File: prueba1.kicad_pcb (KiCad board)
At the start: 2 copper layers, 98.5 x 97 mm, 20 parts, among them J1 GY_63, J2 BMI_270, J3 CMPS2, J4 SHT21, J5 ATGM336H, J7 Cargador, J8 KG200Z, J9 BATERIA, Q1 MCP1702-3302E_TO, U1 TEMP_BAT, U2 DC-DC_STEP_UP

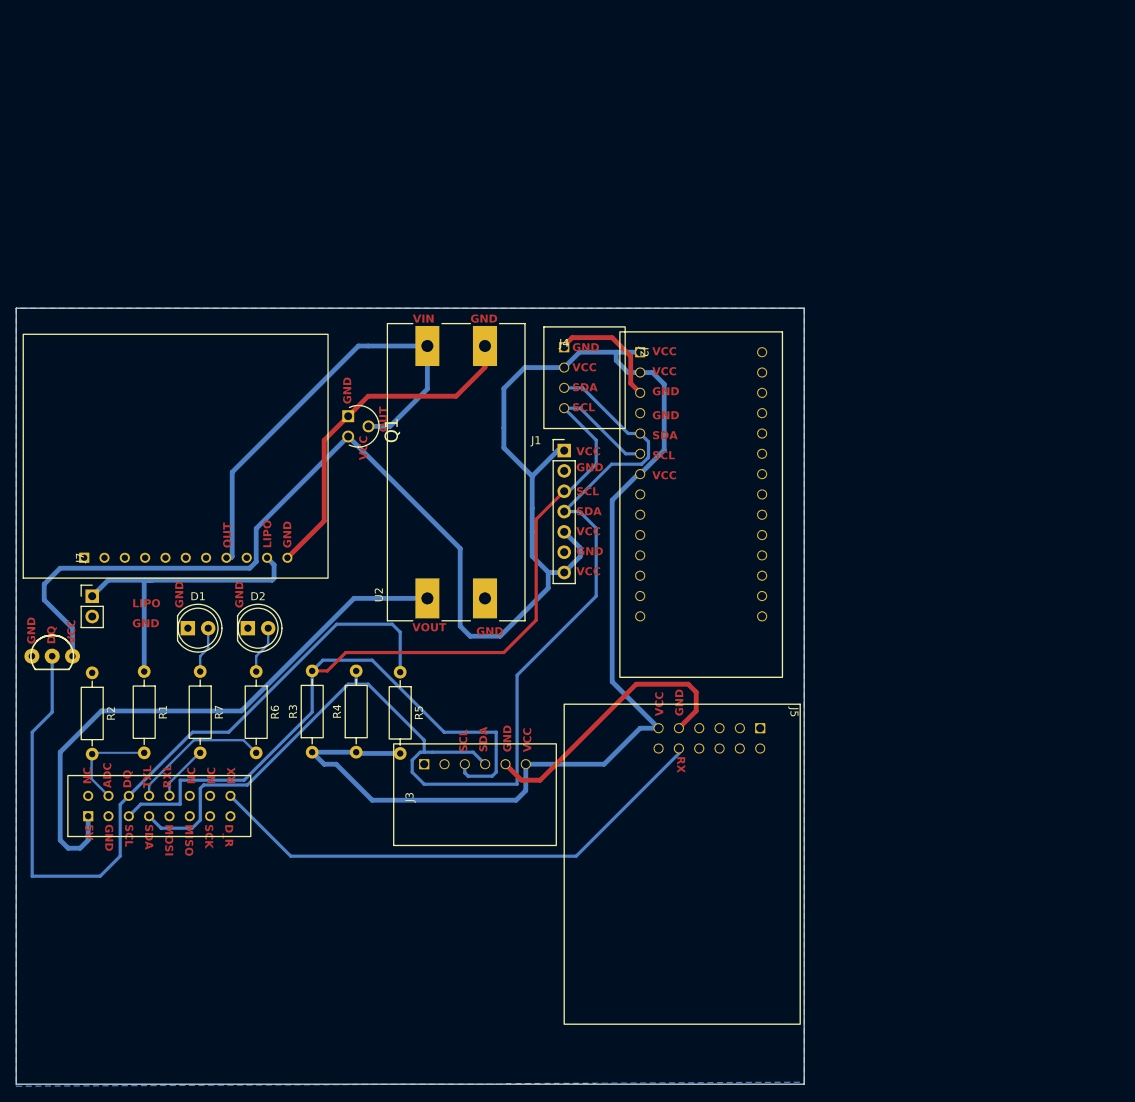
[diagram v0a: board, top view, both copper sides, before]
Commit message: pcb terminada
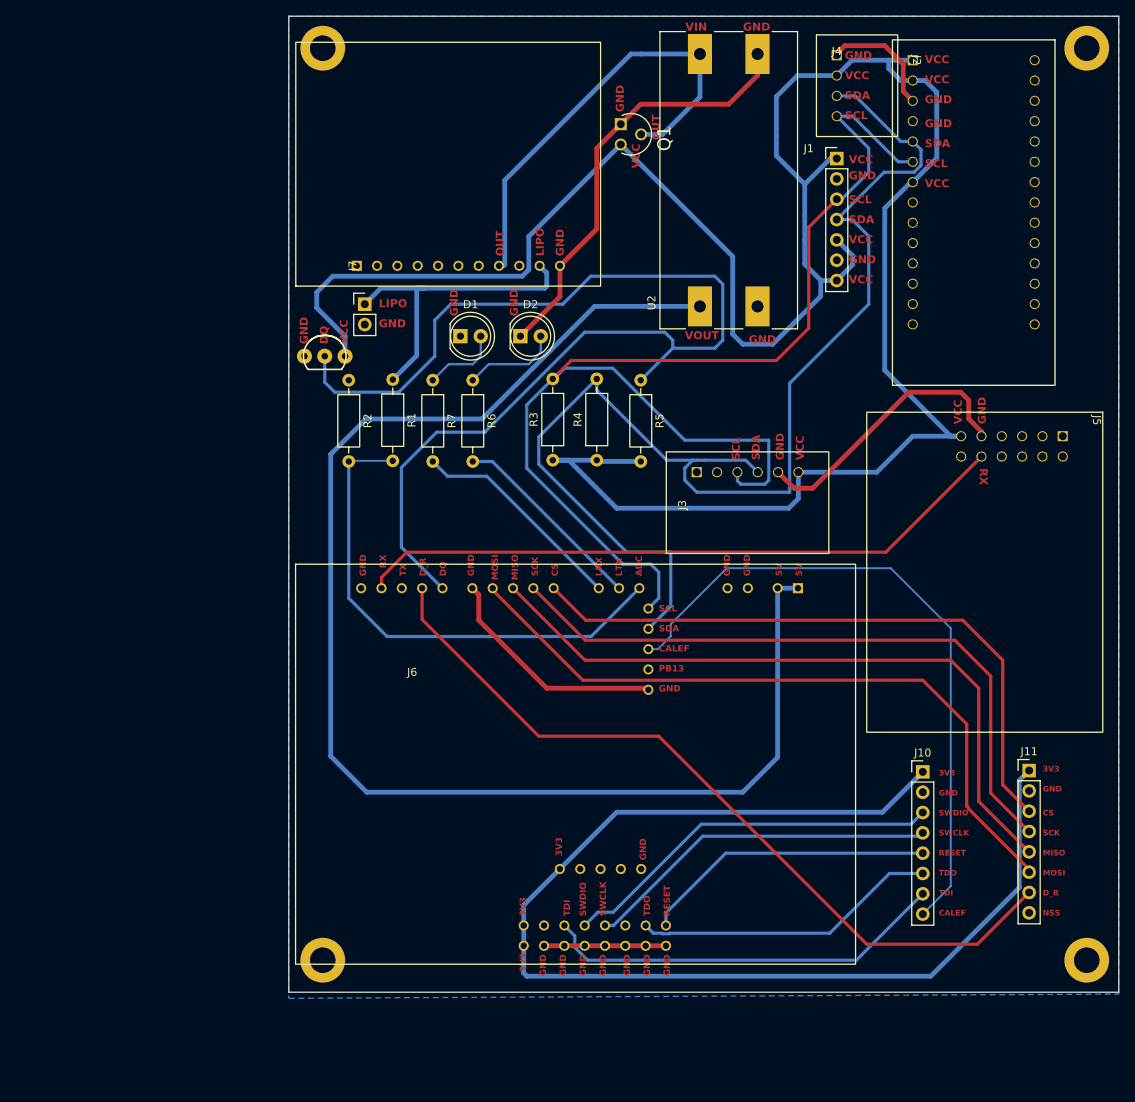
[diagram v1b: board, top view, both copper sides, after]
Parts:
- removed J8: KG200Z, madeinhome:kg200z
- added J10: Conn_01x08_Pin, Connector_PinHeader_2.54mm:PinHeader_1x08_P2.54mm_Vertical, F.Cu at (146.3, 125.5)
- added J11: Conn_01x08_Pin, Connector_PinHeader_2.54mm:PinHeader_1x08_P2.54mm_Vertical, F.Cu at (159.6, 125.3)
- added J6: KG200Z, pines:socket_cont, F.Cu at (67.9, 102.5)
- added REF**: MountingHole_3.2mm_Pad, MountingHole:MountingHole_3.2mm_M3_DIN965_Pad, F.Cu at (71.3, 149.0)
- added REF**: MountingHole_3.2mm_Pad, MountingHole:MountingHole_3.2mm_M3_DIN965_Pad, F.Cu at (166.8, 149.0)
- added REF**: MountingHole_3.2mm_Pad, MountingHole:MountingHole_3.2mm_M3_DIN965_Pad, F.Cu at (166.8, 35.0)
- added REF**: MountingHole_3.2mm_Pad, MountingHole:MountingHole_3.2mm_M3_DIN965_Pad, F.Cu at (71.3, 35.0)
- moved J5 52.6 mm to (163.8, 83.5)
- moved U1 50.7 mm to (71.6, 73.5)
- moved Q1 49.9 mm to (111.1, 47.0)
- moved D1 49.9 mm to (88.5, 71.0)
- moved D2 49.9 mm to (96.0, 71.0)
- moved J1 49.9 mm to (135.6, 48.8)
- moved J2 49.9 mm to (145.1, 36.5)
- moved J3 49.9 mm to (118.1, 95.6)
- moved J4 49.9 mm to (135.6, 35.9)
- moved J7 49.9 mm to (75.6, 62.2)
- moved J9 49.9 mm to (76.6, 67.0)
- moved U2 49.9 mm to (122.1, 51.5)
- moved R2 48.6 mm to (74.6, 76.5)
- moved R1 47.9 mm to (80.1, 76.4)
- moved R3 47.3 mm to (100.1, 86.5)
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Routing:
- net /VDD_3V3: track 0.00 -> 147.1 mm
- net /5V: track 73.2 -> 175.8 mm
- net /D_R: track 0.00 -> 99.3 mm
- net /MOSI: track 0.00 -> 88.2 mm
- net /MISO: track 0.00 -> 86.5 mm
- net /CALEF: track 0.00 -> 83.2 mm
- net /SCK: track 0.00 -> 83.1 mm
- net /CS: track 0.00 -> 80.1 mm
- net /GND: track 93.6 -> 148.5 mm
- net /ADC: track 12.7 -> 63.7 mm
- net /TDI: track 0.00 -> 50.9 mm
- net /SWDIO: track 0.00 -> 48.1 mm
- net /DQ: track 96.8 -> 141.4 mm
- net /SWCLK: track 0.00 -> 44.5 mm
- net /TDO: track 0.00 -> 38.2 mm
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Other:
- board size 98.5 x 97 mm -> 103.8 x 122 mm
- board text added: "3V3"
- board text added: "CALEF"
- board text added: "CS"
- board text added: "LRX"
- board text added: "LTX"
- board text added: "NSS"
- board text added: "PB13"
- board text added: "RESET"
- board text added: "SWCLK"
- board text added: "SWDIO"
- board text added: "TDI"
- board text added: "TDO"
- board text added: "TX"
- board text removed: "NC"
- board text removed: "RXL"
- board text removed: "TXL"
